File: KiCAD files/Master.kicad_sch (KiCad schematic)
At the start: 24 parts, among them SW1 EG1271A, SW2 EG1271A, SW3 EG1271A, SW4 EG1271A, U4 NUCLEO64-F446RE

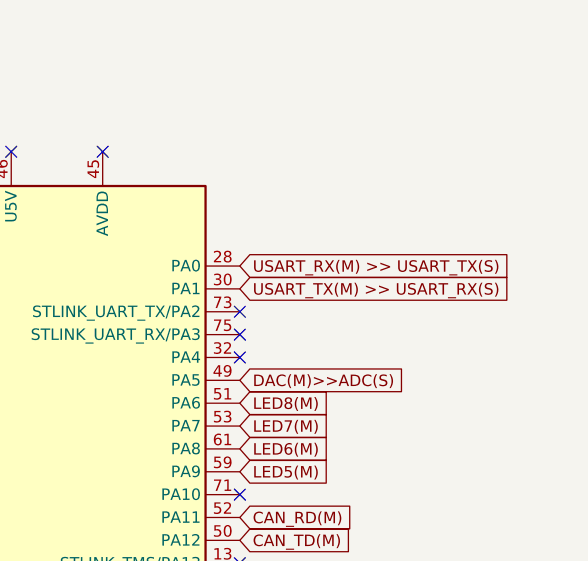
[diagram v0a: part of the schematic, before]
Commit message: update
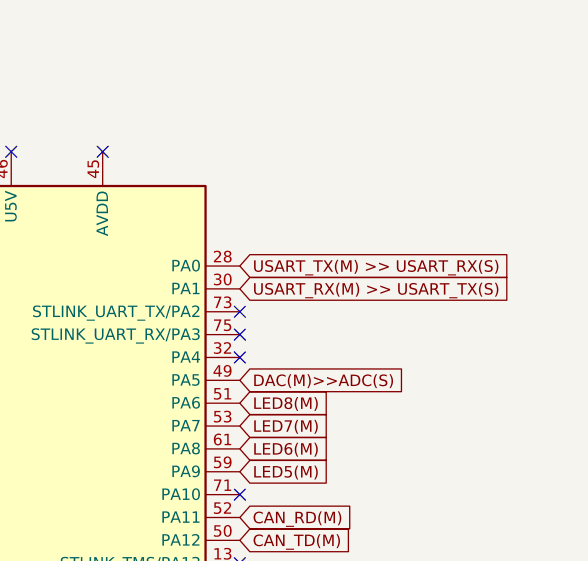
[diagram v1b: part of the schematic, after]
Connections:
- net USART_RX(M) >> USART_TX(S): now also U4.30 (PA1); no longer U4.28 (PA0)
- net USART_TX(M) >> USART_RX(S): now also U4.28 (PA0); no longer U4.30 (PA1)
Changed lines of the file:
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@@
     )
   )
-  (global_label "USART_TX(M) >> USART_RX(S)" (shape input) (at 169.545 55.88 0) (fields_autoplaced)
+  (global_label "USART_TX(M) >> USART_RX(S)" (shape input) (at 169.545 53.34 0) (fields_autoplaced)
     (effects (font (size 1.27 1.27)) (justify left))
-    (property "Intersheetrefs" "${INTERSHEET_REFS}" (at 201.9821 55.88 0)
+    (property "Intersheetrefs" "${INTERSHEET_REFS}" (at 201.9821 53.34 0)
       (effects (font (size 1.27 1.27)) (justify left) hide)
     )
@@
     )
   )
-  (global_label "USART_RX(M) >> USART_TX(S)" (shape input) (at 169.545 53.34 0) (fields_autoplaced)
+  (global_label "USART_RX(M) >> USART_TX(S)" (shape input) (at 169.545 55.88 0) (fields_autoplaced)
     (effects (font (size 1.27 1.27)) (justify left))
-    (property "Intersheetrefs" "${INTERSHEET_REFS}" (at 201.9821 53.34 0)
+    (property "Intersheetrefs" "${INTERSHEET_REFS}" (at 201.9821 55.88 0)
       (effects (font (size 1.27 1.27)) (justify left) hide)
     )
